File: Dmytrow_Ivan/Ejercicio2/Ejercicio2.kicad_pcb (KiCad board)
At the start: 2 copper layers, 40.6 x 61 mm, 13 parts, among them J1 DB9, U1 SSP3232, U2 AMIS42665TJAA1RG

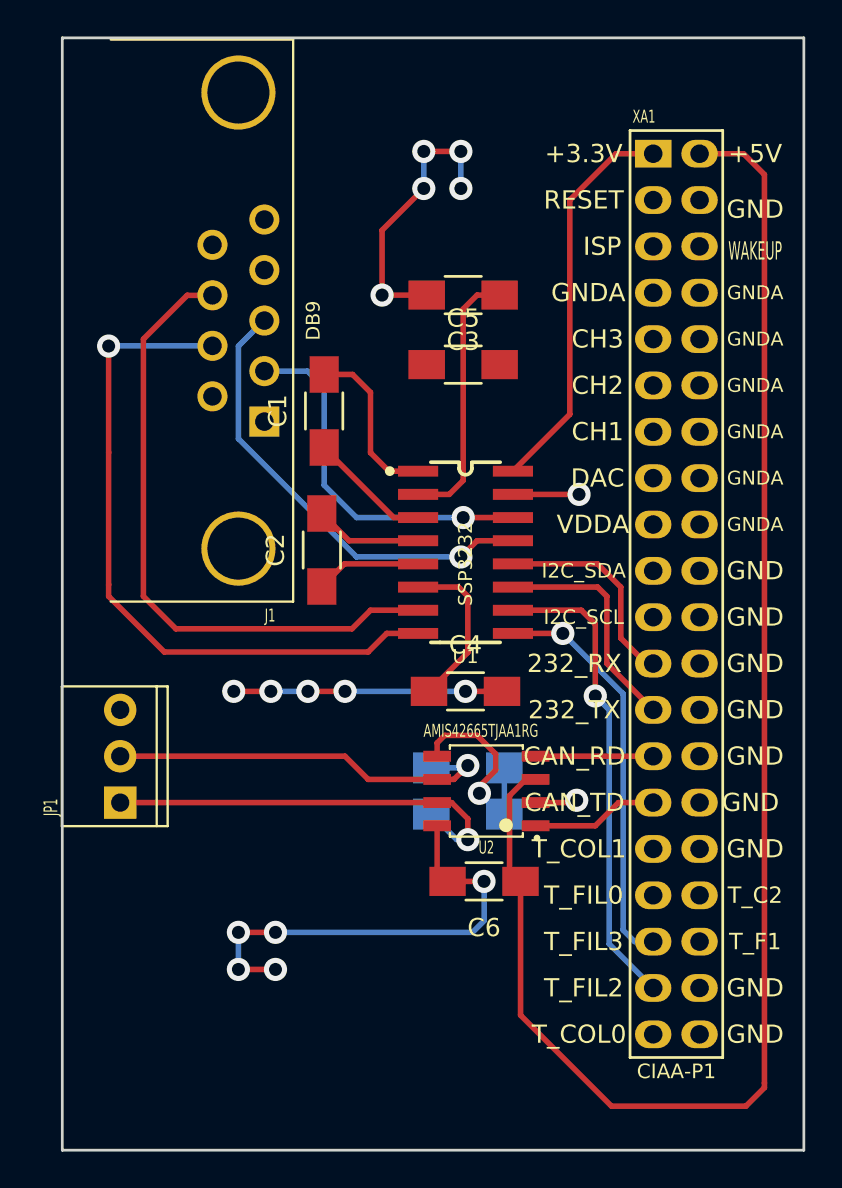
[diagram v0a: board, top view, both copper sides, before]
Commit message: Subo los 3d shapes
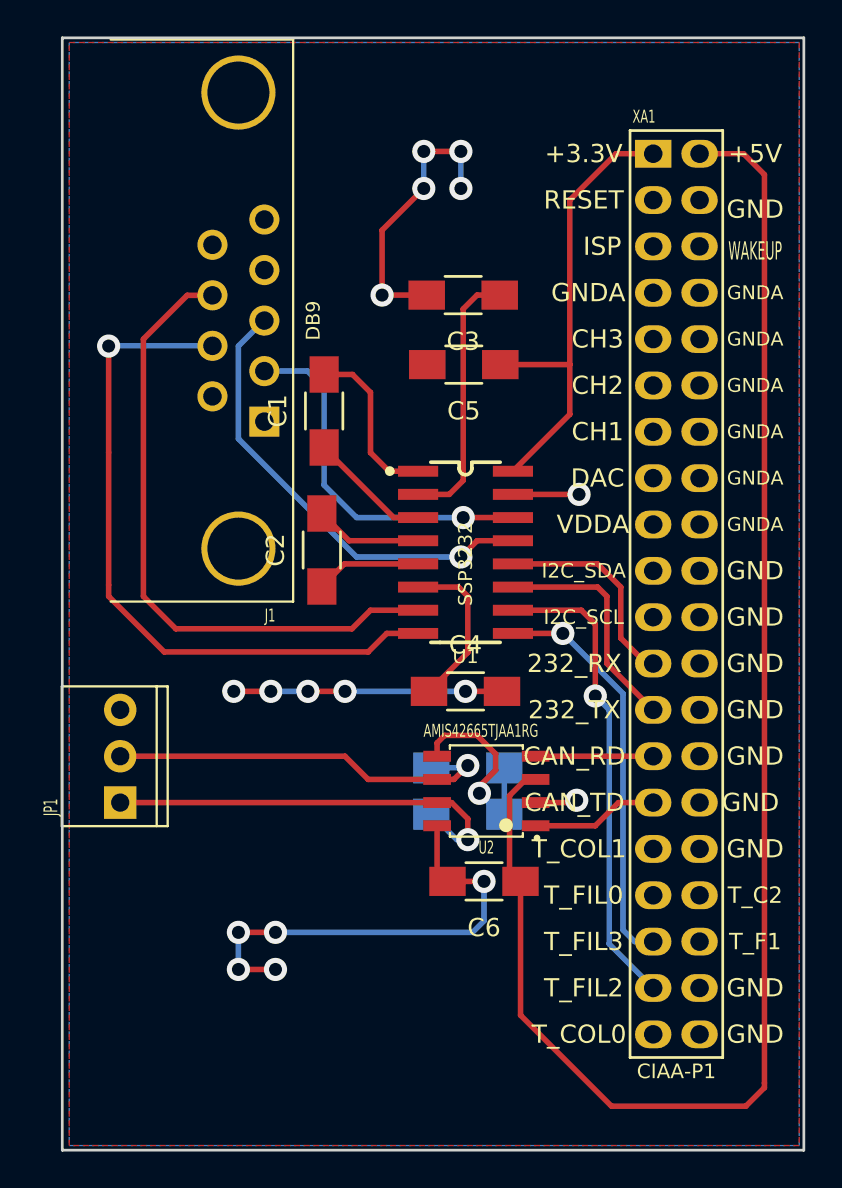
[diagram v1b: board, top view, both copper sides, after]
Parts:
- turned C5 to 0 degrees
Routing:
- net +3.3V: track 21.8 -> 25.6 mm
- added copper zone on B.Cu, net GND
- added copper zone on F.Cu, net GND
